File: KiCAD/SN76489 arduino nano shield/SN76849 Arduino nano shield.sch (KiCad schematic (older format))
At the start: 18 parts, among them J1 Arduino_in, J2 audio_debug, J3 OLED_wit, J4 I2C_in, J5 LOGO, J6 gat1, J7 gat2, J8 geluid_uit, U1 PCF8574, U2 LM358, U3 SN76489

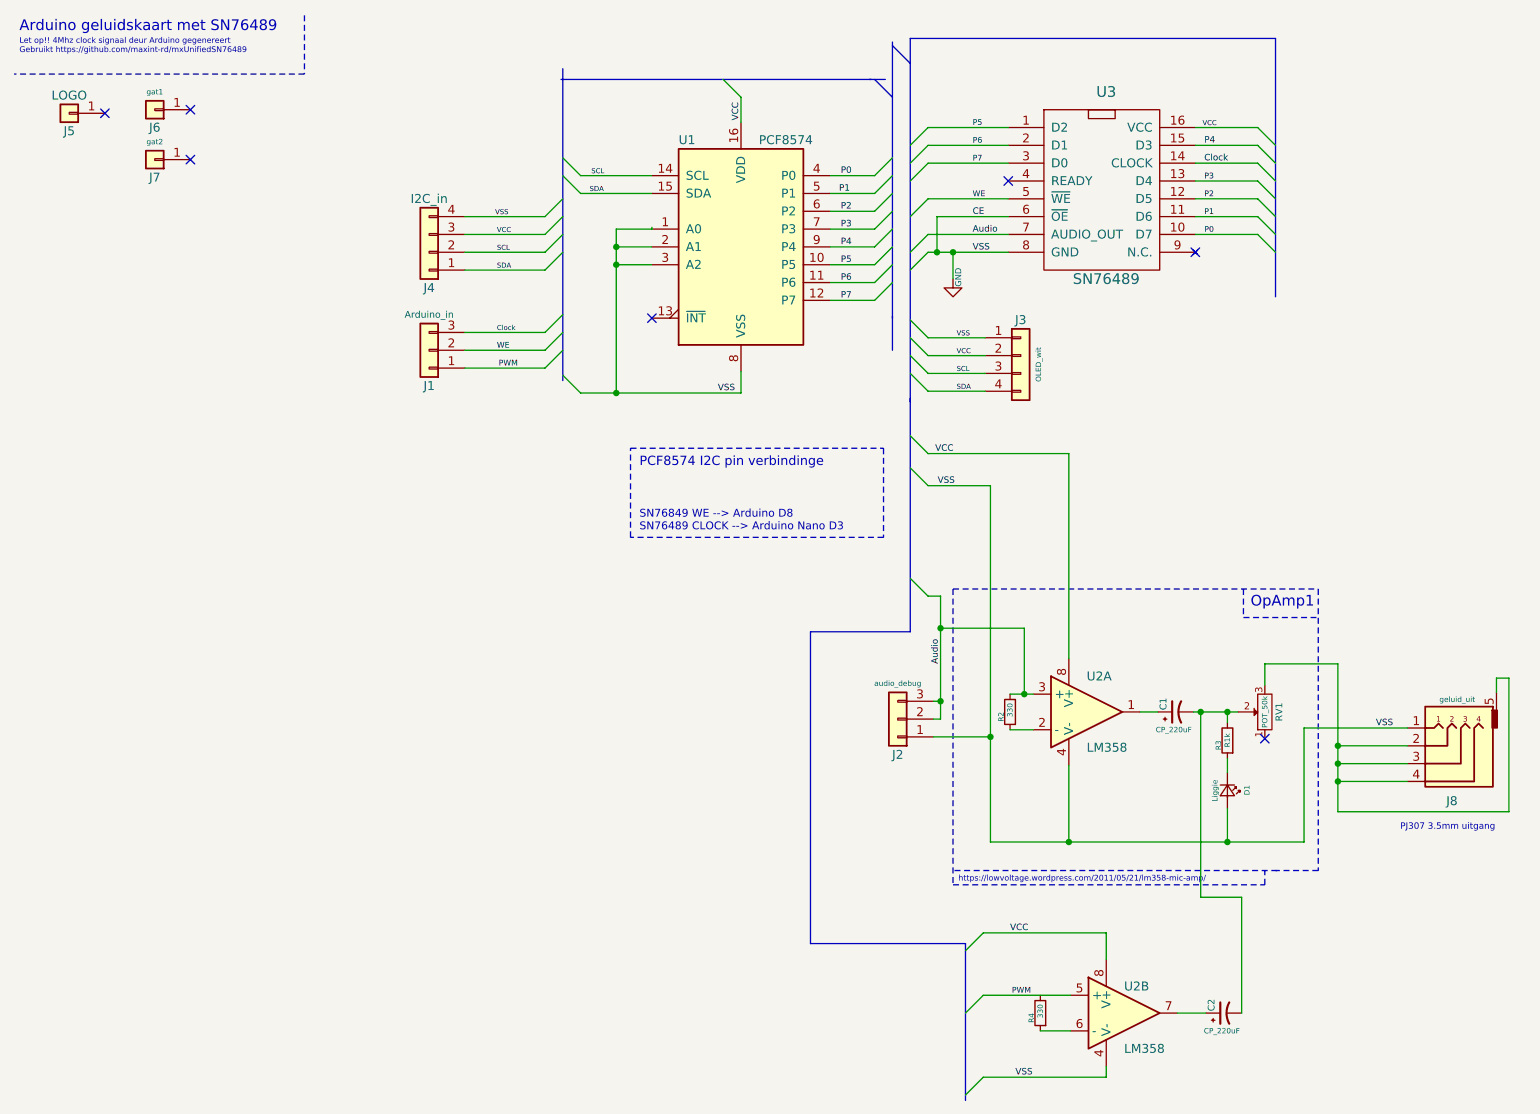
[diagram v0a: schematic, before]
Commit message: update
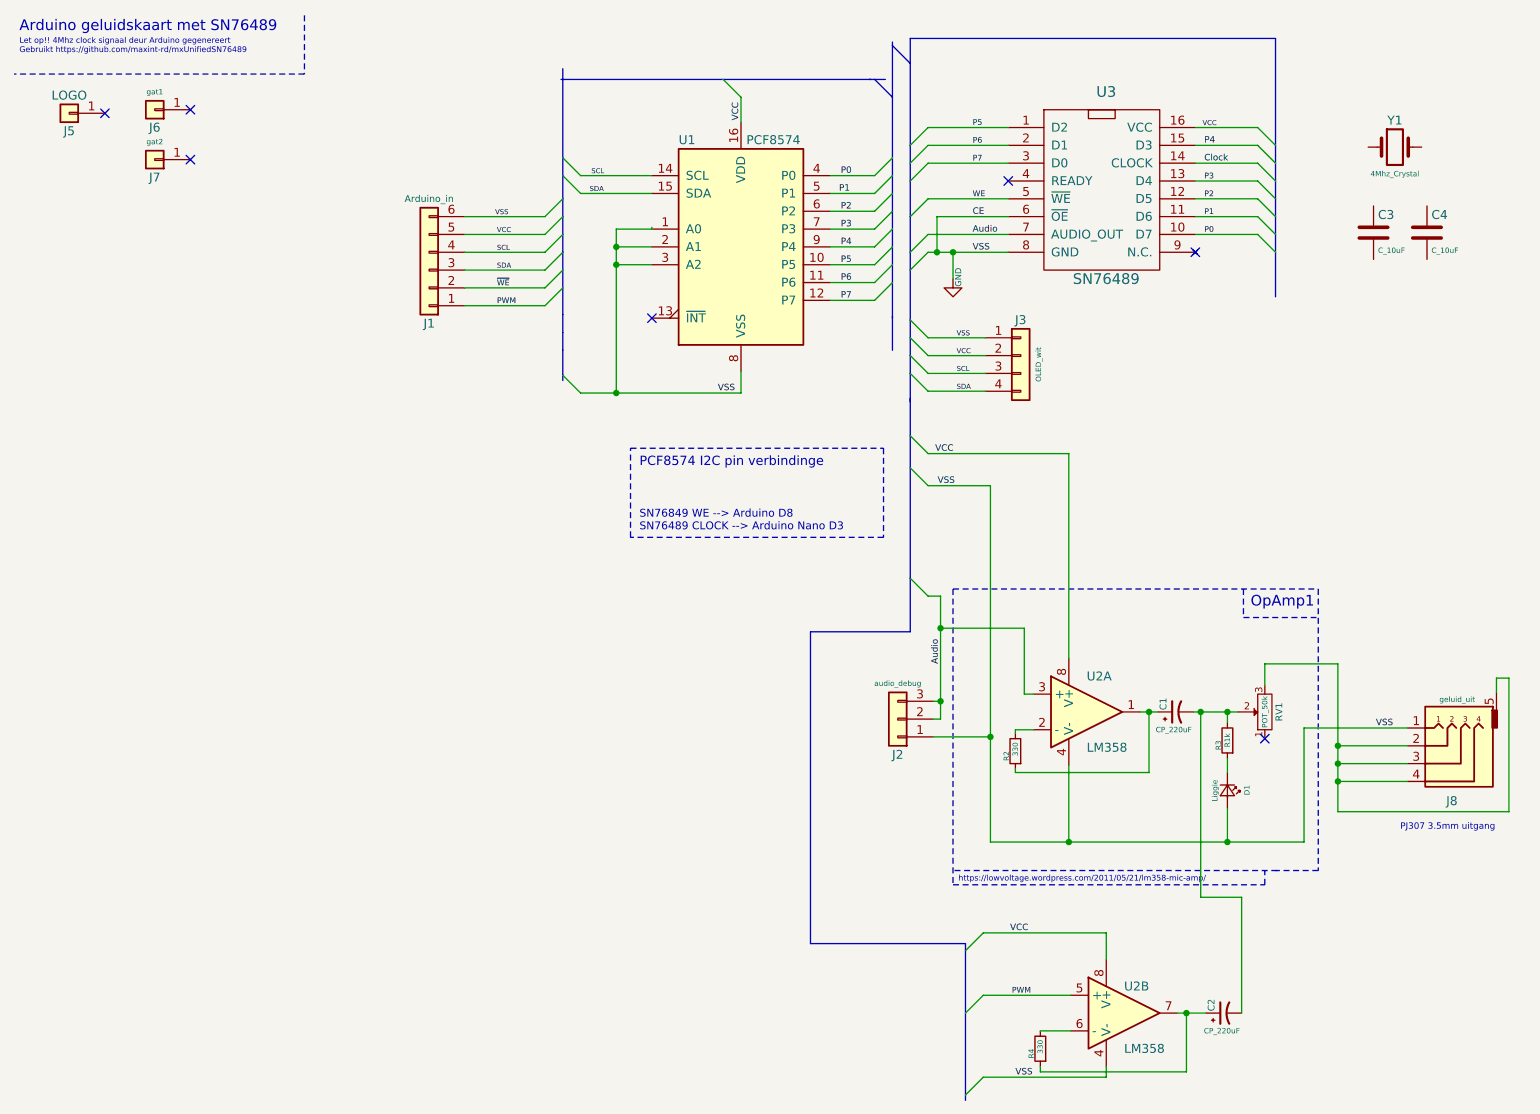
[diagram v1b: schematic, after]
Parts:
- removed J1: Arduino_in, Pin_Headers:Pin_Header_Angled_1x04_Pitch2.54mm, symbol Conn_01x03
- removed J4: I2C_in, Pin_Headers:Pin_Header_Angled_1x04_Pitch2.54mm, symbol Conn_01x04
- added C3, C4: C_10uF, symbol C
- added J1: Arduino_in, symbol Conn_01x06
- added Y1: 4Mhz_Crystal, symbol Crystal
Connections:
- net Audio: no longer R2.2
- net GND: now also J1.6 (Pin_6)
- net PWM: now also J1.1 (Pin_1)
- net SCL: now also J1.4 (Pin_4)
- net SDA: now also J1.3 (Pin_3)
- net VCC: now also J1.5 (Pin_5)
- net at R2.1: now also C1.1, U2.1; no longer U2.2 (-)
- net at U2.6 (-): now also R4.2; no longer R4.1
- net at C2.1, U2.7: now also R4.1
- new net: R2.2, U2.2 (-)
- new net ~WE: J1.2 (Pin_2)
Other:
- moved on the sheet: R2, R4

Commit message: Upgrade project naar KiCAD 4.0.0
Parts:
- C1, C2: symbol CP1_Small -> Device:CP1_Small
- C3, C4: symbol C -> Device:C
- D1: symbol LED_Small -> Device:LED_Small
- J1: symbol Conn_01x06 -> conn:Conn_01x06
- J2: symbol Conn_01x03 -> conn:Conn_01x03
- J3: symbol Conn_01x04 -> conn:Conn_01x04
- J5, J6, J7: symbol Conn_01x01 -> conn:Conn_01x01
- J8: symbol Audio-Jack-5 -> conn:Audio-Jack-5
- R2, R3, R4: symbol R_Small -> Device:R_Small
- RV1: symbol POT-RESCUE-SN76849_Arduino_nano_shield -> SN76849-Arduino-nano-shield-rescue:POT-RESCUE-SN76849_Arduino_nano_shield
- U1: symbol PCF8574 -> philips:PCF8574
- U2: symbol LM358 -> linear:LM358
- U3: symbol SN76489 -> easylab4kids:SN76489
- Y1: symbol Crystal -> Device:Crystal
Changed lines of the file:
@@
-EESchema Schematic File Version 2
-LIBS:SN76849 Arduino nano shield-rescue
-LIBS:power
-LIBS:device
-LIBS:transistors
-LIBS:conn
-LIBS:linear
-LIBS:regul
-LIBS:74xx
-LIBS:cmos4000
-LIBS:adc-dac
-LIBS:memory
-LIBS:xilinx
-LIBS:microcontrollers
-LIBS:dsp
-LIBS:microchip
-LIBS:analog_switches
-LIBS:motorola
-LIBS:texas
-LIBS:intel
-LIBS:audio
-LIBS:interface
-LIBS:digital-audio
-LIBS:philips
-LIBS:display
-LIBS:cypress
-LIBS:siliconi
-LIBS:opto
-LIBS:atmel
-LIBS:contrib
-LIBS:valves
-LIBS:arduino
-LIBS:easylab4kids
-LIBS:trs_jack
+EESchema Schematic File Version 4
 LIBS:SN76849 Arduino nano shield-cache
-EELAYER 25 0
+EELAYER 26 0
 EELAYER END
 $Descr A4 11693 8268
@@
 NoConn ~ 6050 1410
 $Comp
-L PCF8574 U1
+L philips:PCF8574 U1
 U 1 1 5A7F2E84
 P 4550 1780
@@
 VCC
 $Comp
-L POT-RESCUE-SN76849_Arduino_nano_shield RV1
+L SN76849-Arduino-nano-shield-rescue:POT-RESCUE-SN76849_Arduino_nano_shield RV1
 U 1 1 5A96DB87
 P 7490 4390
@@
 Audio
 $Comp
-L SN76489 U3
+L easylab4kids:SN76489 U3
 U 1 1 5A902B70
 P 6600 1460
@@
 Audio
 $Comp
-L GND #PWR1
+L power:GND #PWR1
 U 1 1 5A9BDD7A
 P 5740 1960
@@
 OpAmp1
 $Comp
-L LED_Small D1
+L Device:LED_Small D1
 U 1 1 5B26D96D
 P 7280 4830
@@
 $EndComp
 $Comp
-L R_Small R3
+L Device:R_Small R3
 U 1 1 5B26DBB3
 P 7280 4550
@@
 $EndComp
 $Comp
-L Conn_01x01 J5
+L conn:Conn_01x01 J5
 U 1 1 5B26F111
 P 780 1030
@@
 $EndComp
 $Comp
-L Conn_01x01 J6
+L conn:Conn_01x01 J6
 U 1 1 5B26F3ED
 P 1260 1010
@@
 $EndComp
 $Comp
-L Conn_01x01 J7
+L conn:Conn_01x01 J7
 U 1 1 5B26F4E1
 P 1260 1290
@@
 $EndComp
 $Comp
-L Audio-Jack-5 J8
+L conn:Audio-Jack-5 J8
 U 1 1 5B26D965
 P 8490 4680
@@
 $EndComp
 $Comp
-L CP1_Small C1
+L Device:CP1_Small C1
 U 1 1 5B26BD41
 P 6990 4390
@@
 NoConn ~ 980  1030
 $Comp
-L Conn_01x04 J3
+L conn:Conn_01x04 J3
 U 1 1 5B43DC64
 P 6120 2390
@@
 	7100 1710 7450 1710
 Wire Bus Line
-	7550 610  7550 1210
-Wire Bus Line
-	7550 1210 7550 1310
-Wire Bus Line
-	7550 1310 7550 1410
-Wire Bus Line
-	7550 1410 7550 1510
-Wire Bus Line
-	7550 1510 7550 1610
-Wire Bus Line
-	7550 1610 7550 1710
-Wire Bus Line
-	7550 1710 7550 1810
-Wire Bus Line
-	7550 1810 7550 2060
-Wire Bus Line
 	5500 610  7550 610
 Wire Wire Line
@@
 Wire Wire Line
 	3650 1380 4050 1380
-Wire Bus Line
-	5400 630  5400 650
-Wire Bus Line
-	5400 650  5400 940
-Wire Bus Line
-	5400 940  5400 1280
-Wire Bus Line
-	5400 1280 5400 1380
-Wire Bus Line
-	5400 1380 5400 1480
-Wire Bus Line
-	5400 1480 5400 1580
-Wire Bus Line
-	5400 1580 5400 1680
-Wire Bus Line
-	5400 1680 5400 1780
-Wire Bus Line
-	5400 1780 5400 1880
-Wire Bus Line
-	5400 1880 5400 1980
-Wire Bus Line
-	5400 1980 5400 2180
-Wire Bus Line
-	3550 780  3550 1280
-Wire Bus Line
-	3550 1280 3550 1380
-Wire Bus Line
-	3550 1380 3550 1510
-Wire Bus Line
-	3550 1510 3550 1610
-Wire Bus Line
-	3550 1610 3550 1710
-Wire Bus Line
-	3550 1710 3550 1810
-Wire Bus Line
-	3550 1810 3550 2160
-Wire Bus Line
-	3550 2160 3550 2260
-Wire Bus Line
-	3550 2260 3550 2360
-Wire Bus Line
-	3550 2360 3550 2500
-Wire Bus Line
-	3550 2500 3550 2530
 Wire Wire Line
 	3000 2010 3450 2010
@@
 Wire Wire Line
 	5300 2080 5050 2080
-Wire Bus Line
-	3540 840  4450 840
-Wire Bus Line
-	4450 840  5280 840
-Wire Bus Line
-	5270 840  5300 840
-Wire Bus Line
-	5300 840  5360 840
-Wire Bus Line
-	5400 2170 5400 2360
 Wire Notes Line
 	3930 2910 5350 2910
@@
 	3850 1880 3850 2600
 Connection ~ 3850 2600
-Wire Notes Line
-	7560 5280 5740 5280
 Wire Wire Line
 	5600 1710 6050 1710
@@
 Wire Notes Line
 	7790 3700 7790 5280
-Wire Notes Line
-	7790 5280 7550 5280
 Wire Notes Line
 	5740 3700 5740 5360
@@
 Wire Wire Line
 	5670 4330 5670 4430
-Wire Bus Line
-	5500 610  5500 750
-Wire Bus Line
-	5500 750  5500 1210
-Wire Bus Line
-	5500 1210 5500 1310
-Wire Bus Line
-	5500 1310 5500 1410
-Wire Bus Line
-	5500 1410 5500 1610
-Wire Bus Line
-	5500 1610 5500 1810
-Wire Bus Line
-	5500 1810 5500 1910
-Wire Bus Line
-	5500 1910 5500 2190
-Wire Bus Line
-	5500 2190 5500 2290
-Wire Bus Line
-	5500 2290 5500 2390
-Wire Bus Line
-	5500 2390 5500 2490
-Wire Bus Line
-	5500 2490 5500 2650
 Wire Wire Line
 	5600 3740 5670 3740
-Wire Bus Line
-	5500 2630 5500 2840
-Wire Bus Line
-	5500 2840 5500 3020
-Wire Bus Line
-	5500 3020 5500 3640
-Wire Bus Line
-	5500 3640 5500 3940
 Wire Wire Line
 	5650 1610 5650 1810
@@
 	5920 2590 5600 2590
 $Comp
-L R_Small R2
+L Device:R_Small R2
 U 1 1 5A9B7BDC
 P 6090 4610
@@
 $EndComp
 $Comp
-L LM358 U2
+L linear:LM358 U2
 U 1 1 5B4FA1EF
 P 6490 4390
@@
 $EndComp
 $Comp
-L LM358 U2
+L linear:LM358 U2
 U 2 1 5B4FA234
 P 6700 6080
@@
 Wire Bus Line
 	4940 5690 5810 5690
-Wire Bus Line
-	5810 5690 5810 5730
-Wire Bus Line
-	5810 5730 5810 6080
-Wire Bus Line
-	5810 6080 5810 6540
-Wire Bus Line
-	5810 6540 5810 6570
 Entry Wire Line
 	5810 5730 5910 5630
@@
 Connection ~ 5950 4530
 $Comp
-L R_Small R4
+L Device:R_Small R4
 U 1 1 5B510C1C
 P 6230 6280
@@
 Connection ~ 5670 3920
 $Comp
-L CP1_Small C2
+L Device:CP1_Small C2
 U 1 1 5B51233C
 P 7260 6080
@@
 	7130 5430 7130 4390
 $Comp
-L Conn_01x03 J2
+L conn:Conn_01x03 J2
 U 1 1 5B513BA6
 P 5430 4430
@@
 Connection ~ 7050 6080
 $Comp
-L Crystal Y1
+L Device:Crystal Y1
 U 1 1 5B69193B
 P 8220 1220
@@
 $EndComp
 $Comp
-L C C3
+L Device:C C3
 U 1 1 5B691BA9
 P 8100 1700
@@
 $EndComp
 $Comp
-L C C4
+L Device:C C4
 U 1 1 5B691CB5
 P 8400 1700
@@
 $EndComp
 $Comp
-L Conn_01x06 J1
+L conn:Conn_01x06 J1
 U 1 1 5B6930F1
 P 2800 1910
@@
 	-1   0    0    1
 $EndComp
+Wire Notes Line
+	5740 5280 7790 5280
+Wire Bus Line
+	3540 840  5360 840
+Wire Bus Line
+	5810 5690 5810 6570
+Wire Bus Line
+	7550 610  7550 2060
+Wire Bus Line
+	5400 630  5400 2360
+Wire Bus Line
+	3550 780  3550 2530
+Wire Bus Line
+	5500 610  5500 3940
 $EndSCHEMATC

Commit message: versie 20180905 0.7.06
LM358 opAmp wasverwyderd,
Dip-14 Xtal clock 4Mhz toegevoegd.
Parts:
- removed C2: CP_220uF, Capacitors_THT:CP_Radial_D8.0mm_P2.50mm, symbol Device:CP1_Small
- removed C3, C4: C_10uF, symbol Device:C
- removed J1: Arduino_in, symbol conn:Conn_01x06
- removed R2, R4: 330, w_pth_resistors:RC03, symbol Device:R_Small
- removed U2: LM358, w_pth_circuits:dil_8-300_socket, symbol linear:LM358
- removed Y1: 4Mhz_Crystal, symbol Device:Crystal
- added J1: Arduino_in, Pin_Headers:Pin_Header_Angled_1x05_Pitch2.54mm, symbol conn:Conn_01x05
- added X1: CLK_DIP14_4Mhz, Oscillators:Oscillator_DIP-14_LargePads, symbol Oscillator:CXO_DIP14
- C1: footprint Capacitors_THT:CP_Radial_D8.0mm_P2.50mm -> Capacitors_THT:CP_Radial_D10.0mm_P3.50mm
- RV1: footprint w_pth_resistors:trimmer_ecp_ca9-v10 -> w_pth_resistors:trimmer_ecp_ca9-h2,5
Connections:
- net labels removed: PWM, WE
- wire segments 110 -> 91
- no-connect marks 7 -> 8
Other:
- note removed: "OpAmp1"
- note removed: "https://lowvoltage.wordpress.com/2011/05/21/lm358-mic-amp/"
